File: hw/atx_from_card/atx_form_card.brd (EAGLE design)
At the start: 45 x 80 mm, 31 parts

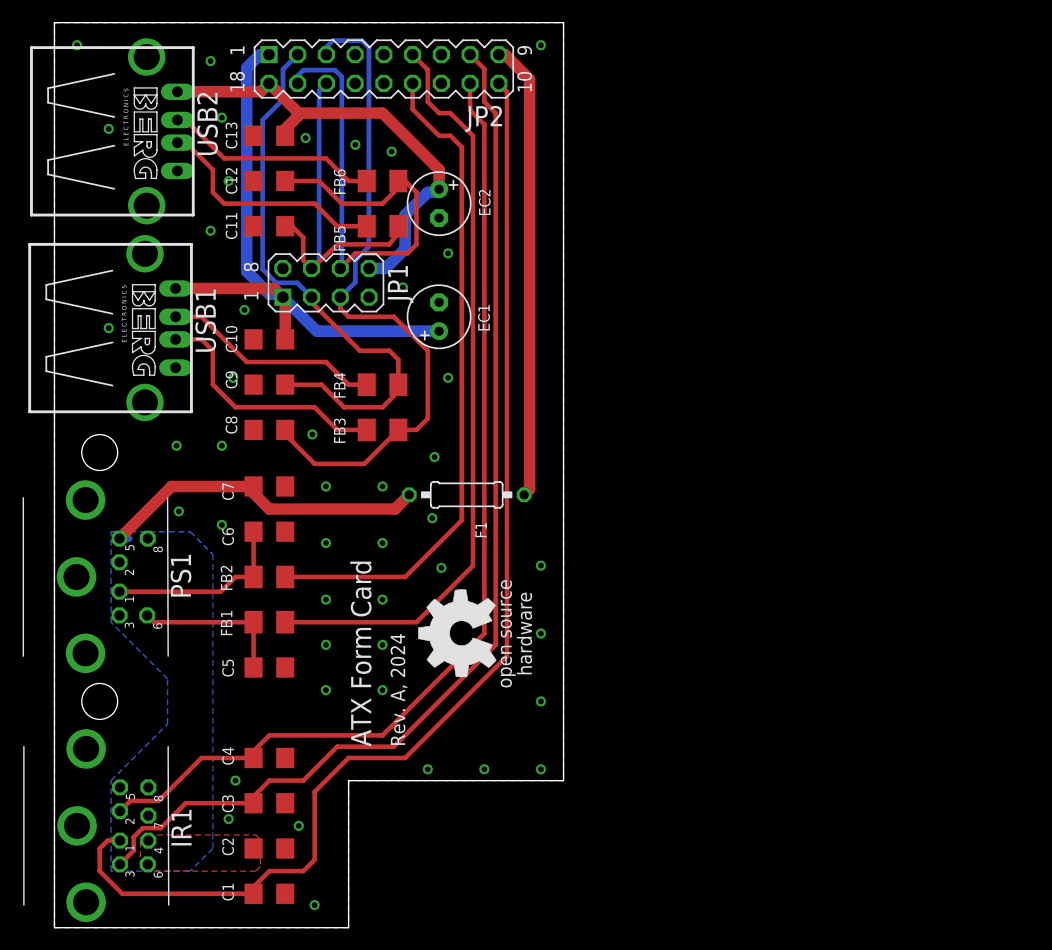
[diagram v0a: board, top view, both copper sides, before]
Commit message: Rev. D of the board. Added more documentation.
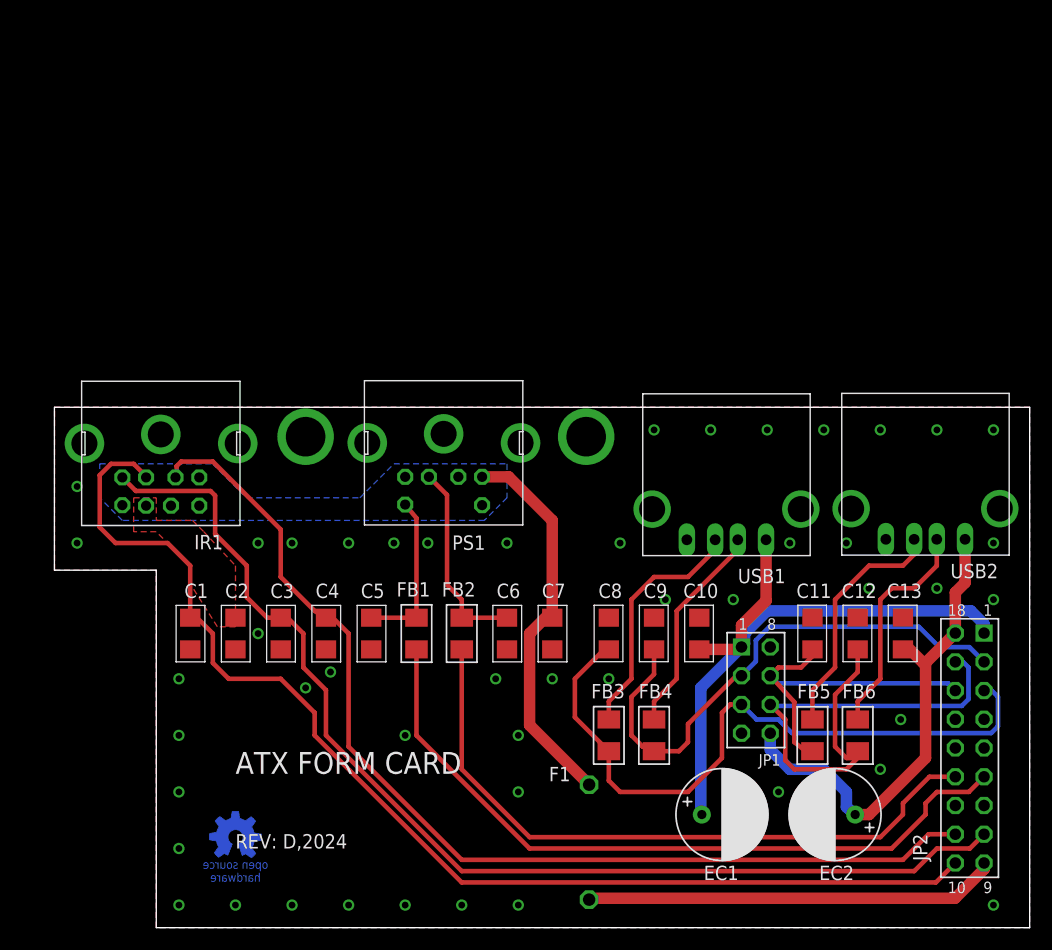
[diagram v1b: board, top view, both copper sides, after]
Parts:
- removed U$1: (no value), oshw_custom:OSHW_8MM
- removed U$3, U$4: (no value), special-drill:DRILL_0.1250
- added U$2: (no value), oshw_custom:OSHW_5MM
- C1, C10, C11, C12, C13, C2, C3, C4, C5, C6, C7, C8, C9: device resistor:C3216 -> resistor-custom:C3216
- EC1, EC2: device resistor:E2,5-6 -> resistor-custom:E3,5-8
- F1: device resistor:0207/10 -> resistor-custom:0207/10
- FB1, FB2, FB3, FB4, FB5, FB6: device resistor:M3216 -> resistor-custom:M3216
- USB1, USB2: device con-berg:PN87520-S -> con-berg-custom:PN87520-S
- moved JP2 79.3 mm to (80.9, 15.9), turned to 0 degrees
- moved USB2 76.5 mm to (77.0, 37.0), turned to 180 degrees
- moved C13 71.2 mm to (75.0, 26.0), turned to 90 degrees
- moved C12 65.6 mm to (71.0, 26.0), turned to 90 degrees
- moved FB6 64.5 mm to (71.0, 17.0), turned to 270 degrees
- moved EC2 64.4 mm to (69.0, 10.0), turned to 180 degrees
- moved C11 60.0 mm to (67.0, 26.0), turned to 90 degrees
- moved FB5 58.9 mm to (67.0, 17.0), turned to 270 degrees
- moved USB1 53.8 mm to (59.4, 37.0), turned to 180 degrees
- moved JP1 52.3 mm to (62.0, 21.0), turned to 0 degrees
- moved EC1 50.6 mm to (59.0, 10.0), turned to 0 degrees
- moved C10 46.0 mm to (57.0, 26.0), turned to 90 degrees
- moved C9 40.5 mm to (53.0, 26.0), turned to 90 degrees
- moved FB4 39.2 mm to (53.0, 17.0), turned to 270 degrees
- moved IR1 35.4 mm to (9.40, 43.6), turned to 0 degrees
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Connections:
- net VCC: no longer IR1.6
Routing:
- net IRLO: track 88.2 -> 93.8 mm
- net VCC: track 30.1 -> 34.5 mm
- net N$8: track 40.6 -> 36.5 mm
- net IRHI: track 96.6 -> 99.7 mm
- net VBUS1: track 53.2 -> 55.3 mm
- net DATA1-: track 50.0 -> 48.0 mm
- net VBUS2: track 41.8 -> 43.8 mm
- net MSECLK: track 66.6 -> 65.1 mm
- net N$2: track 16.4 -> 17.7 mm
- net IROUT: track 105.6 -> 104.4 mm
- net N$3: track 19.0 -> 20.0 mm
- net DATA2+: track 32.3 -> 31.3 mm
- net DATA2-: track 49.1 -> 48.2 mm
- net MSEDATA: track 58.7 -> 59.5 mm
- net N$6: track 13.6 -> 14.4 mm
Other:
- board size 45 x 80 mm -> 86.2 x 46 mm
- board text added: "ATX FORM CARD"
- board text added: "REV: D,2024"
- board text removed: "ATX Form Card"
- board text removed: "Rev. A, 2024"
